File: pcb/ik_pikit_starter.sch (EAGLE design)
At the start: 30 parts, among them U1 QRE1113, U2 MCP9700SMD

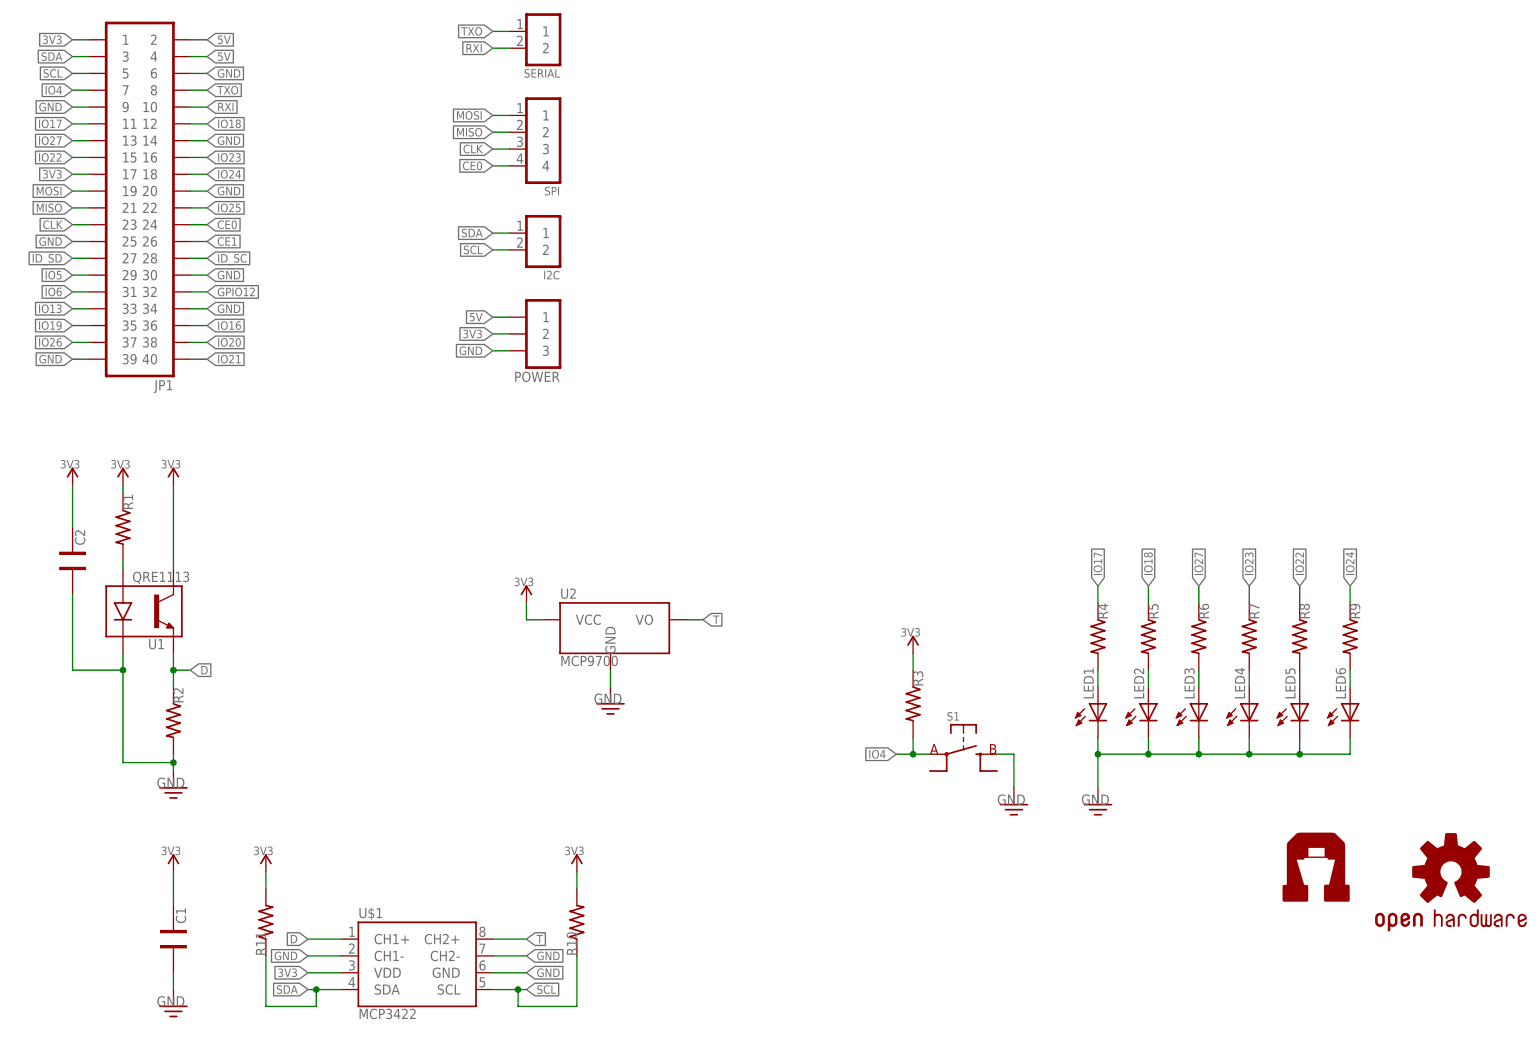
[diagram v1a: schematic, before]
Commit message: adding values
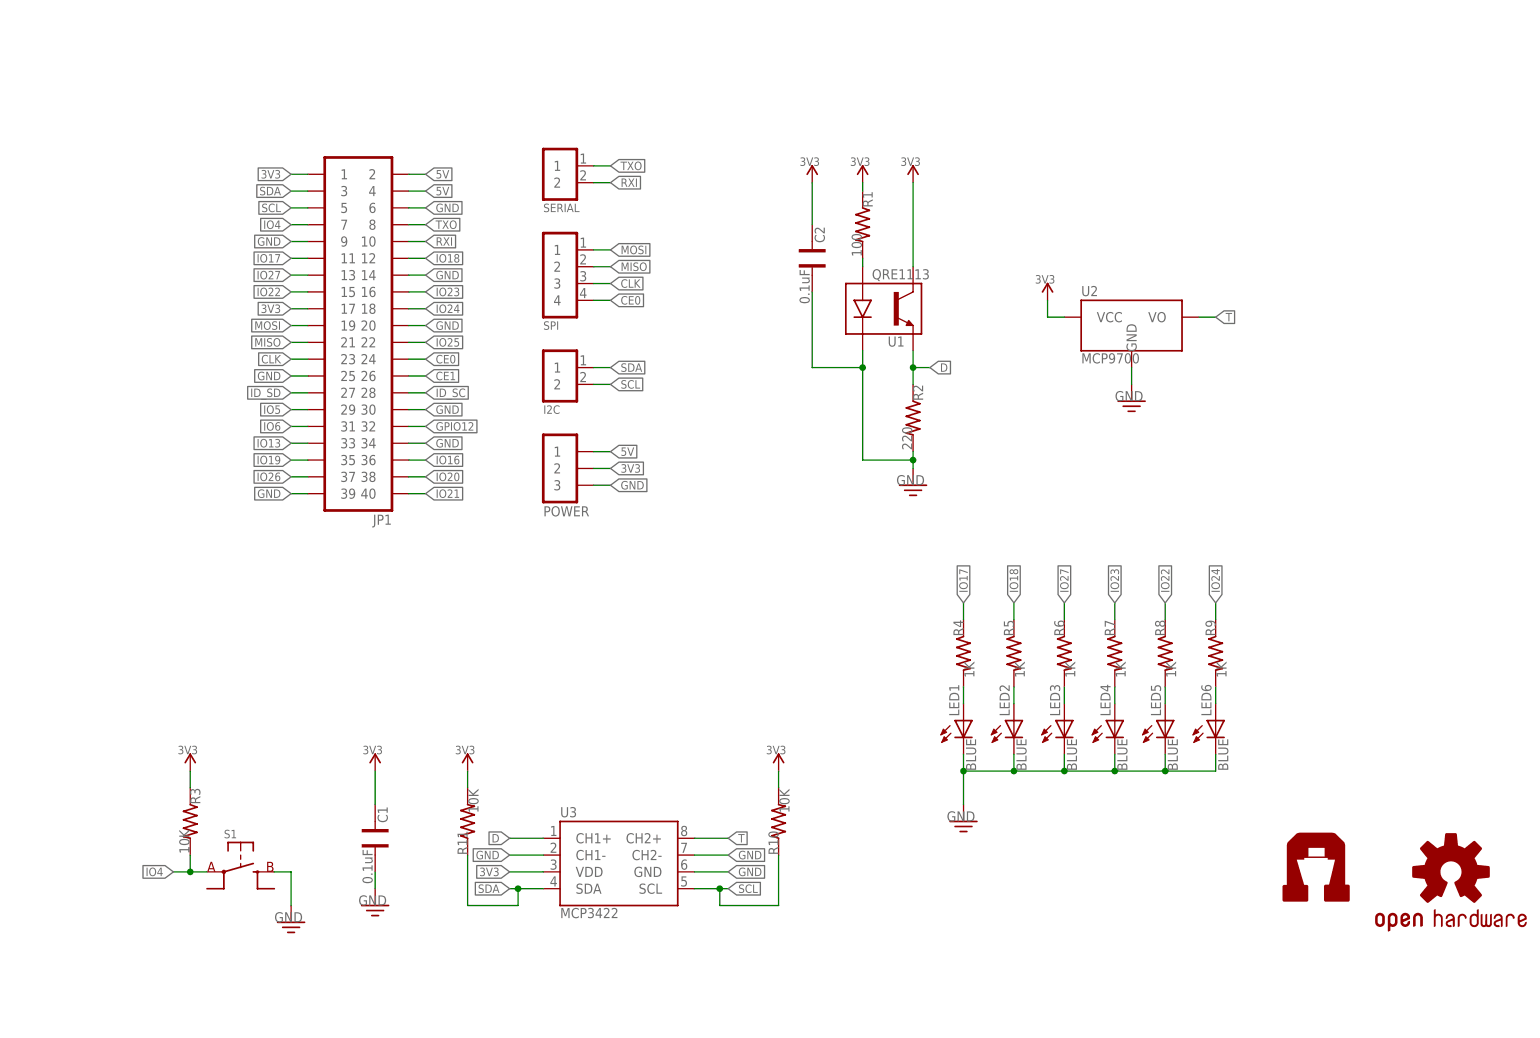
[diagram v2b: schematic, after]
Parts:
- removed U$1: MCP3422, Ai_IC:MCP3422
- added U3: MCP3422, Ai_IC:MCP3422
- C1, C2: value (none) -> 0.1uF
- LED1, LED2, LED3, LED4, LED5, LED6: value (none) -> BLUE
- R1: value (none) -> 100
- R10, R11, R3: value (none) -> 10K
- R2: value (none) -> 220
- R4, R5, R6, R7, R8, R9: value (none) -> 1K
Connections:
- net 3V3: now also U3.VDD; no longer U$1.VDD
- net D: now also U3.CH1+; no longer U$1.CH1+
- net GND: now also U3.CH1-, U3.CH2-, U3.GND; no longer U$1.CH1-, U$1.CH2-, U$1.GND
- net SCL: now also U3.SCL; no longer U$1.SCL
- net SDA: now also U3.SDA; no longer U$1.SDA
- net T: now also U3.CH2+; no longer U$1.CH2+
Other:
- moved on the sheet: C1, C2, I2C, JP1, LED1, LED2, LED3, LED4, LED5, LED6, POWER, R1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
